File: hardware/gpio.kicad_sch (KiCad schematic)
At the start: 13 parts, among them U4 GateMate-CCGM1A1

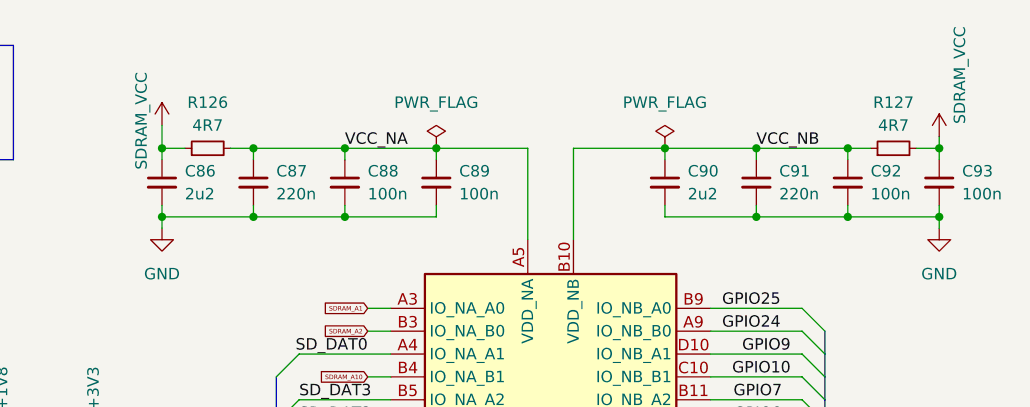
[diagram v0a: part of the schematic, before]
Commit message: CleanUP
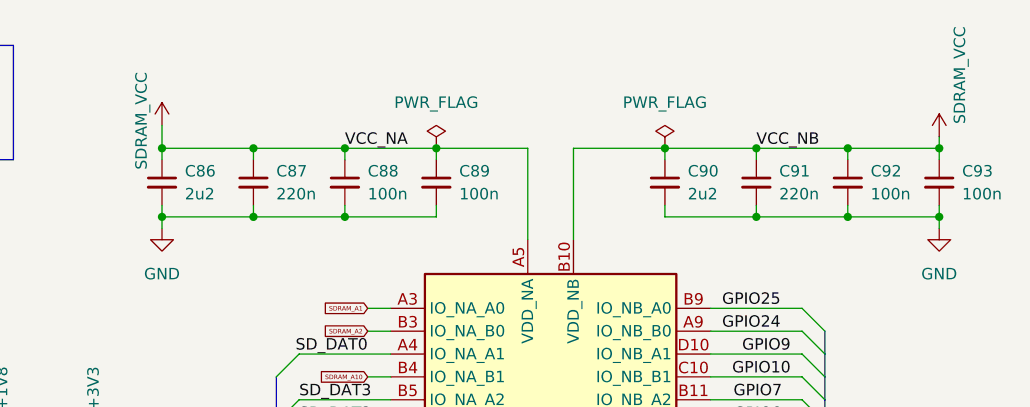
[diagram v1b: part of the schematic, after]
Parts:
- removed R126, R127: 4R7, Resistor_SMD:R_0402_1005Metric, symbol Device:R_Small
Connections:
- net VCC_NA is gone; now on net SDRAM_VCC: C87.1, C88.1, C89.1, U4.A5 (VDD_NA), U4.B7 (VDD_NA), U4.E6 (VDD_NA), U4.E8 (VDD_NA), U4.F7 (VDD_NA)
- net VCC_NB is gone; now on net SDRAM_VCC: C90.1, C91.1, C92.1, U4.B10 (VDD_NB), U4.B13 (VDD_NB), U4.E10 (VDD_NB), U4.E12 (VDD_NB), U4.F11 (VDD_NB)
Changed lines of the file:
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@@
 	(wire
 		(pts
-			(xy 109.22 38.1) (xy 111.76 38.1)
+			(xy 109.22 38.1) (xy 119.38 38.1)
 		)
 		(stroke
@@
 	(wire
 		(pts
-			(xy 185.42 38.1) (xy 187.96 38.1)
+			(xy 185.42 38.1) (xy 195.58 38.1)
 		)
 		(stroke
@@
 	(wire
 		(pts
-			(xy 193.04 38.1) (xy 195.58 38.1)
-		)
-		(stroke
-			(width 0)
-			(type default)
-		)
-	)
-	(wire
-		(pts
 			(xy 195.58 38.1) (xy 195.58 39.37)
 		)
@@
 		(pts
 			(xy 121.92 73.66) (xy 121.92 76.2)
-		)
-		(stroke
-			(width 0)
-			(type default)
-		)
-	)
-	(wire
-		(pts
-			(xy 116.84 38.1) (xy 119.38 38.1)
 		)
 		(stroke
@@
 			)
 			(justify left)
-		)
-	)
-	(symbol
-		(lib_id "Device:R_Small")
-		(at 190.5 38.1 90)
-		(unit 1)
-		(exclude_from_sim no)
-		(in_bom yes)
-		(on_board yes)
-		(dnp no)
-		(property "Reference" "R127"
-			(at 190.5 33.02 90)
-			(effects
-				(font
-					(size 1.27 1.27)
-				)
-			)
-		)
-		(property "Value" "4R7"
-			(at 190.5 35.56 90)
-			(effects
-				(font
-					(size 1.27 1.27)
-				)
-			)
-		)
-		(property "Footprint" "Resistor_SMD:R_0402_1005Metric"
-			(at 190.5 38.1 0)
-			(effects
-				(font
-					(size 1.27 1.27)
-				)
-				(hide yes)
-			)
-		)
-		(property "Datasheet" "~"
-			(at 190.5 38.1 0)
-			(effects
-				(font
-					(size 1.27 1.27)
-				)
-				(hide yes)
-			)
-		)
-		(property "Description" "Resistor, small symbol"
-			(at 190.5 38.1 0)
-			(effects
-				(font
-					(size 1.27 1.27)
-				)
-				(hide yes)
-			)
-		)
-		(pin "1"
-		)
-		(pin "2"
-		)
-		(instances
-			(project "ulx5m-gs"
-				(path "/9e5cbfd6-8186-4817-919e-acd256336bc8/a29a432d-2cca-4e45-9947-735d9a1918bd"
-					(reference "R127")
-					(unit 1)
-				)
-			)
 		)
 	)
@@
 					(unit 1)
 				)
-			)
-		)
-	)
-	(symbol
-		(lib_id "Device:R_Small")
-		(at 114.3 38.1 90)
-		(unit 1)
-		(exclude_from_sim no)
-		(in_bom yes)
-		(on_board yes)
-		(dnp no)
-		(property "Reference" "R126"
-			(at 114.3 33.02 90)
-			(effects
-				(font
-					(size 1.27 1.27)
-				)
-			)
-		)
-		(property "Value" "4R7"
-			(at 114.3 35.56 90)
-			(effects
-				(font
-					(size 1.27 1.27)
-				)
-			)
-		)
-		(property "Footprint" "Resistor_SMD:R_0402_1005Metric"
-			(at 114.3 38.1 0)
-			(effects
-				(font
-					(size 1.27 1.27)
-				)
-				(hide yes)
-			)
-		)
-		(property "Datasheet" "~"
-			(at 114.3 38.1 0)
-			(effects
-				(font
-					(size 1.27 1.27)
-				)
-				(hide yes)
-			)
-		)
-		(property "Description" "Resistor, small symbol"
-			(at 114.3 38.1 0)
-			(effects
-				(font
-					(size 1.27 1.27)
-				)
-				(hide yes)
-			)
-		)
-		(pin "1"
-		)
-		(pin "2"
-		)
-		(instances
-			(project "ulx5m-gs"
-				(path "/9e5cbfd6-8186-4817-919e-acd256336bc8/a29a432d-2cca-4e45-9947-735d9a1918bd"
-					(reference "R126")
-					(unit 1)
-				)
